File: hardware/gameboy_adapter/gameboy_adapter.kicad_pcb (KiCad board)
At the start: 2 copper layers, 100 x 33 mm, 7 parts, among them J1 CART SLOT TOP ROW, J2 GBA_Slot, M2_1 Screw_Terminal_01x01, M2_10 Screw_Terminal_01x01, M2_2 Screw_Terminal_01x01, M2_3 Screw_Terminal_01x01, SW1 SW_SPDT

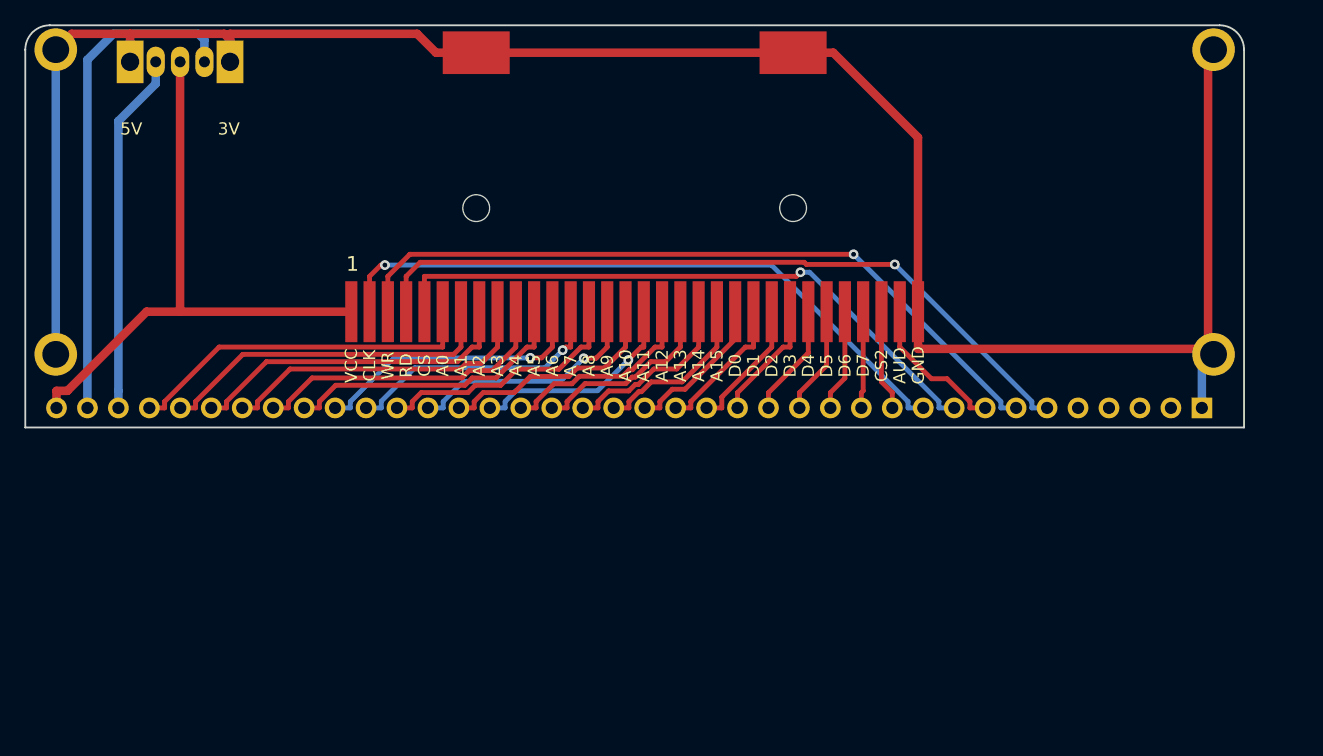
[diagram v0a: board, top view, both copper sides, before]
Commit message: Update gb breakout
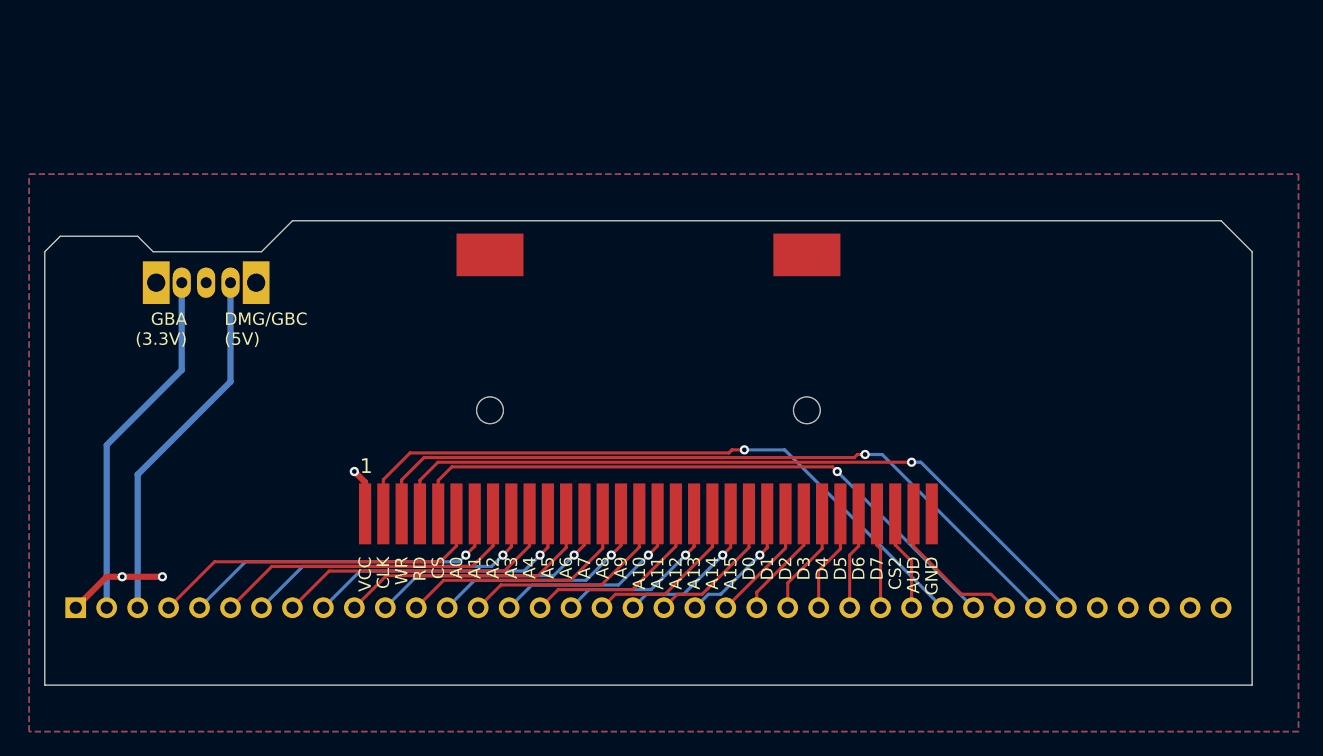
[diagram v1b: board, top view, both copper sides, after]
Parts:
- removed M2_1, M2_10, M2_2, M2_3: Screw_Terminal_01x01, MountingHole:MountingHole_2.2mm_M2_ISO7380_Pad
- J1: footprint Connector_PinSocket_2.54mm:PinSocket_1x38_P2.54mm_Vertical -> Connector_PinHeader_2.54mm:PinHeader_1x38_P2.54mm_Vertical; moved to B.Cu
- J2: footprint !sanni:GBA-SLOT-B -> !OSCR:GBA_Slot
- moved SW1 18.2 mm to (116.8, 71.1)
- moved J2 16.6 mm to (151.1, 85.1)
- moved J1 16.5 mm to (104.1, 97.8), turned to -90 degrees
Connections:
- net D50 renamed MISO
- net D51 renamed MOSI
- net D52 renamed SCK
- net D53 renamed SS
- J1 pad 2: +3V3 -> +3.3V
- SW1 pad 1: +3V3 -> +5V
- SW1 pad 3: +5V -> +3.3V
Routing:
- net GND: track 175.9 -> 0.00 mm
- net +3V3: track 41.1 -> 0.00 mm
- net VCC: track 48.8 -> 12.0 mm, vias 0 -> 3
- net +3.3V: track 0.00 -> 29.2 mm
- net D16: track 53.9 -> 55.1 mm
- net D35: track 10.8 -> 9.73 mm
- net A7: track 22.1 -> 21.0 mm
- net A9: track 20.0 -> 19.0 mm
- net A2: track 27.3 -> 26.3 mm
- net A4: track 25.2 -> 24.2 mm
- net A0: track 29.3 -> 28.3 mm
- net A11: track 17.9 -> 16.9 mm
- net A1: track 28.3 -> 27.3 mm, vias 0 -> 1
- net A12: track 16.9 -> 15.9 mm
- net A13: track 15.8 -> 14.9 mm, vias 0 -> 1
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- added copper zone on B.Cu, net GND
- added copper zone on F.Cu, net GND
- added copper zone on B.Cu, net VCC
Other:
- board size 100 x 33 mm -> 99.1 x 38.1 mm
- board text added: "DMG/GBC (5V)"
- board text added: "GBA (3.3V)"
- board text removed: "3V"
- board text removed: "AUD"
- board text removed: "CLK"
- board text removed: "CS"
- board text removed: "CS2"
- board text removed: "D0"
- board text removed: "D1"
- board text removed: "D2"
- board text removed: "D3"
- board text removed: "D4"
- board text removed: "D5"
- board text removed: "G"
- board text removed: "RD"
- board text removed: "V"
- board text removed: "WR"
